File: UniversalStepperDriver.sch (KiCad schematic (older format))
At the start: 80 parts, among them P1 USB_OTG, P11 CONN_01X04, P12 CONN_01X02, P13 CONN_28BYJ-48, P14 CONN_28BYJ-48, P15 CONN_28BYJ-48, P17 CONN_01X04, P2 CONN_01X02, P3 CONN_01X02, P4 CONN_01X03, P5 Universal_Serial_Connector, P6 CONN_01X06, P7 RPI_header, P8 CONN_01X03, P9 CONN_01X04, SW1 SW_PUSH, SW2 SW_PUSH, SW3 SW_PUSH, U1 STM32F411RE, U2 INA169, U3 MPQ4420, U4 ULN2003V, U5 ULN2003V, Y1 CRYSTAL_SMD_16MHz

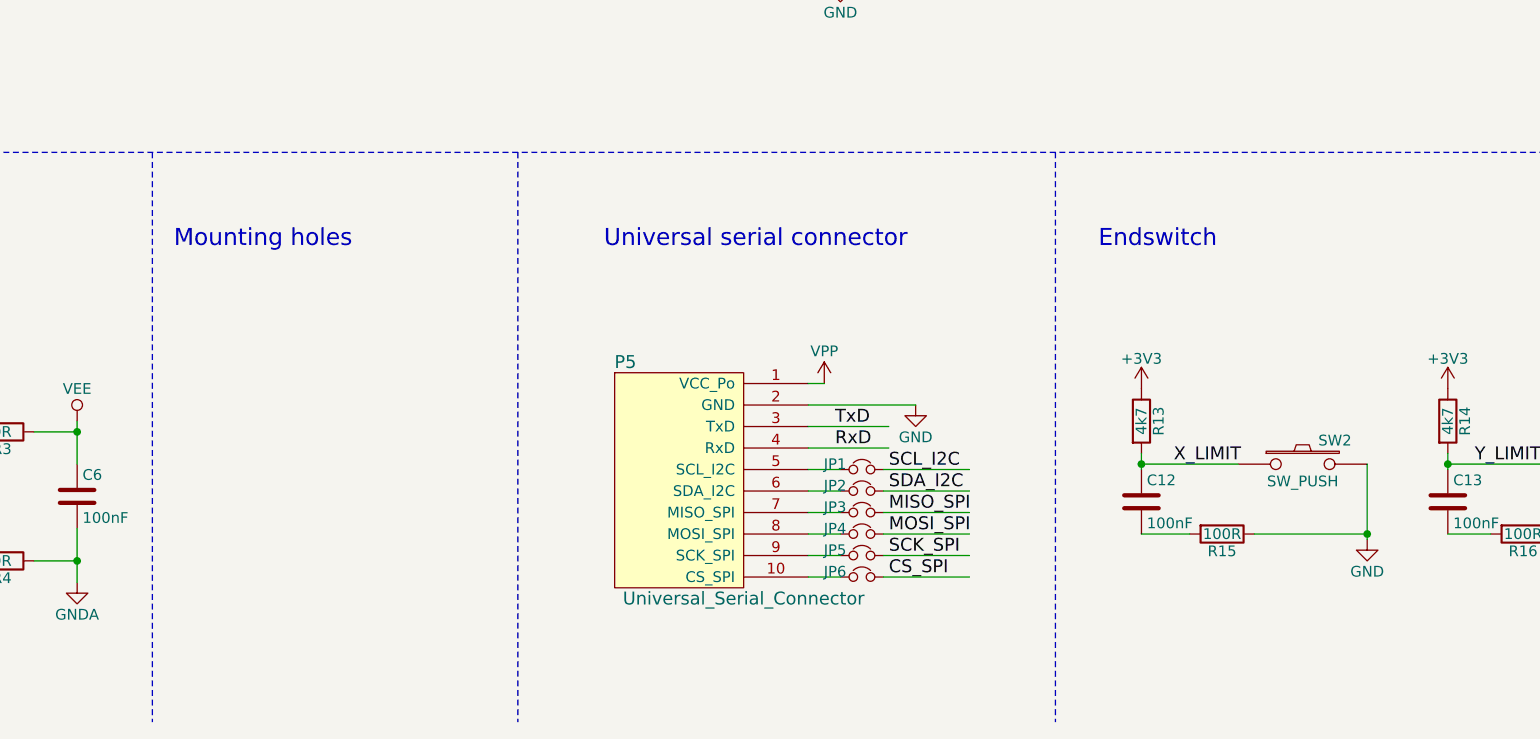
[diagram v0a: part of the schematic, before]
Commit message: rev0.1 board done
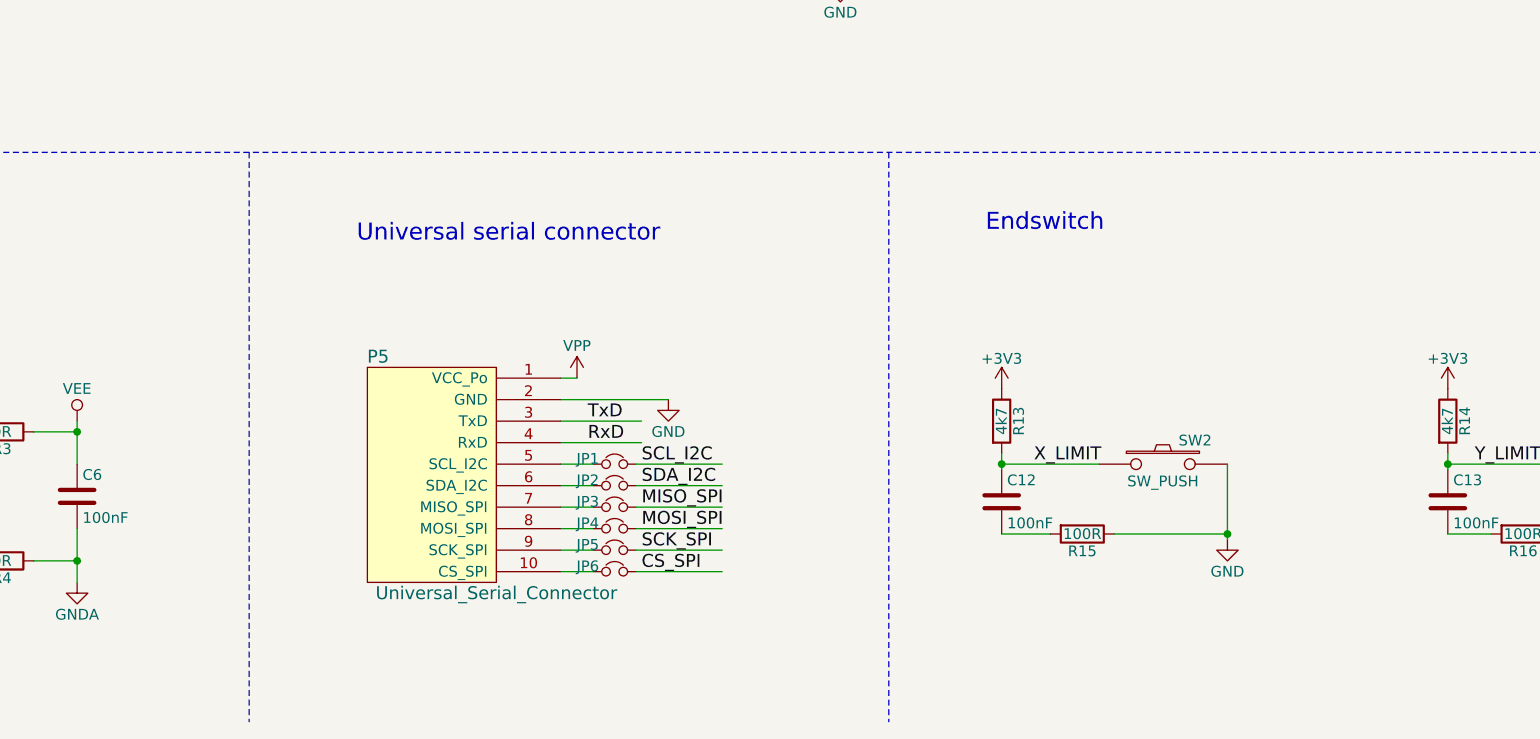
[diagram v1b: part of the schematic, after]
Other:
- note removed: "Mounting holes\n"
- moved on the sheet: C12, JP1, JP2, JP3, JP4, JP5, JP6, P5, R13, R15, SW2
